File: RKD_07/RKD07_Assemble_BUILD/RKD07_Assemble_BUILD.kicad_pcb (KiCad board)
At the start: 2 copper layers, 233.4 x 200 mm, 172 parts, among them J1 Conn_01x02_Socket, J10 Conn_01x04, J11 TRRS, J12 Conn_01x06, J13 Conn_01x06, J14 Conn_01x02_Socket, J2 Conn_01x24, J3 Conn_01x24, J4 Conn_01x24, J5 Qwiic_RA, J6 Qwiic_RA, J7 Conn_01x06, J8 Conn_01x06, J9 Conn_01x04, M3 Mark, M4 Mark, M5 Mark, M6 Mark, M8 Mark, SW1 SW_Push, SW10 SW_Push, SW11 SW_Push, SW12 SW_Push, SW13 SW_Push, SW14 SW_Push, SW15 SW_Push, SW16 SW_Push, SW17 SW_Push, SW18 SW_Push, SW19 SW_Push, SW2 SW_Push, SW20 SW_Push, SW21 SW_Push, SW22 SW_Push, SW23 SW_Push, SW24 SW_Push, SW25 SW_Push, SW26 SW_Push, SW27 SW_Push, SW28 SW_Push, SW29 SW_Push, SW3 SW_Push, SW30 RotaryEncoder_Switch, SW31 SW_Push, SW4 SW_Push, SW5 SW_Push, SW51 SW_Push, SW52 SW_Push, SW53 SW_Push, SW54 SW_Push, SW55 SW_Push, SW56 SW_Push, SW57 SW_Push, SW58 SW_Push, SW59 SW_Push, SW6 SW_Push, SW60 SW_Push, SW61 SW_Push, SW62 SW_Push, SW63 SW_Push, SW64 SW_Push, SW65 SW_Push, SW66 SW_Push, SW67 SW_Push, SW68 SW_Push, SW69 SW_Push, SW7 SW_Push, SW70 SW_Push, SW71 SW_Push, SW72 SW_Push, SW73 SW_Push, SW74 SW_Push, SW75 SW_Push, SW76 SW_Push, SW77 SW_Push, SW78 SW_Push, SW79 SW_Push, SW8 SW_Push, SW80 SW_Push, SW81 SW_Push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

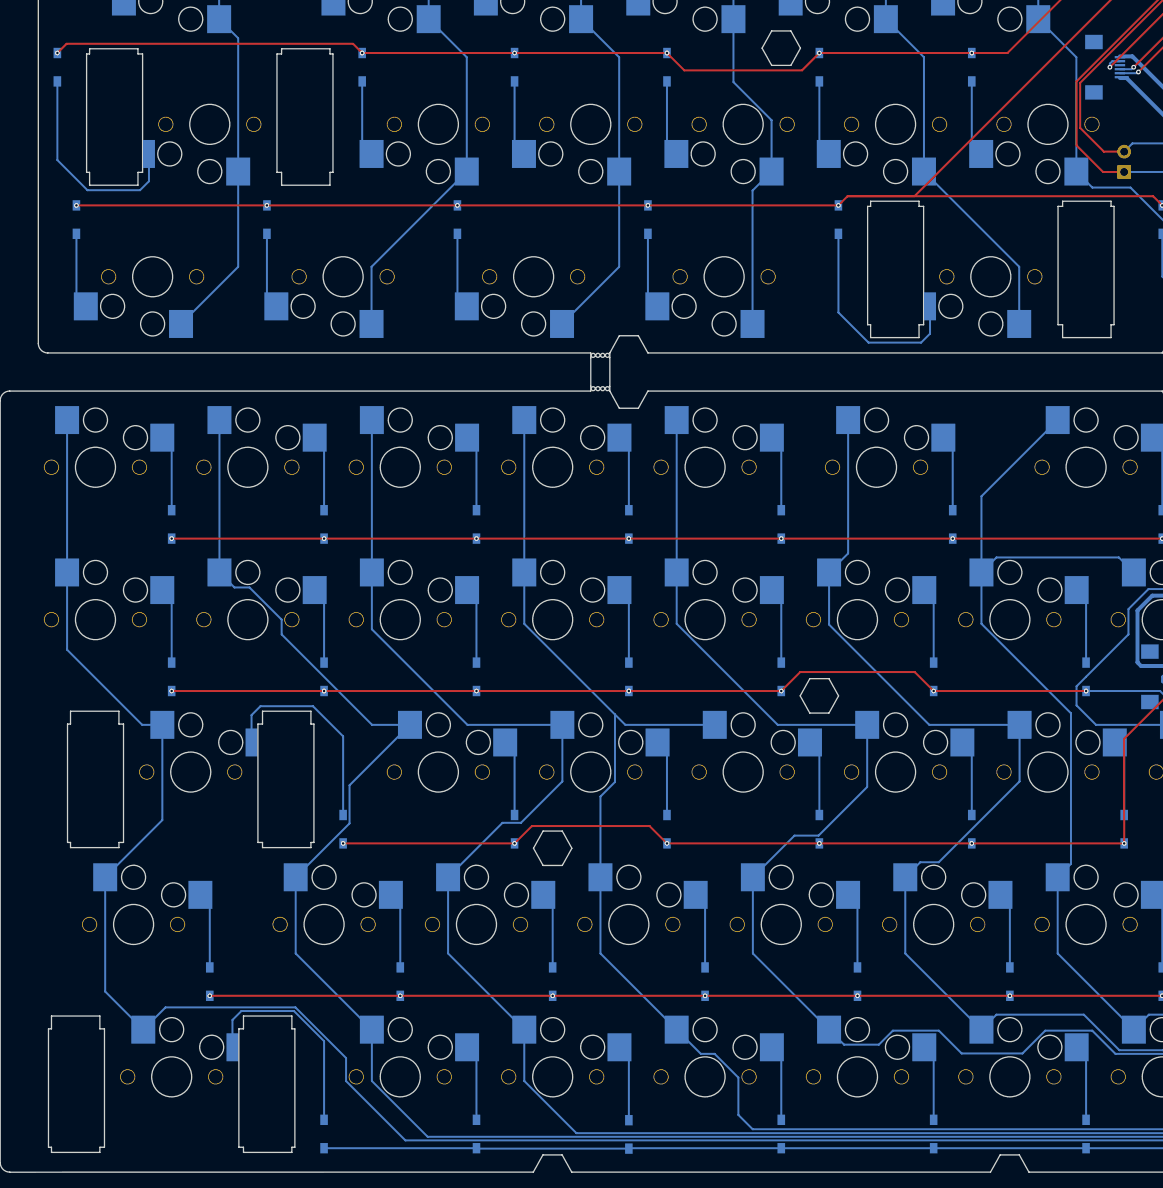
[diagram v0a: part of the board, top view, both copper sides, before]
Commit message: 07 Release調整
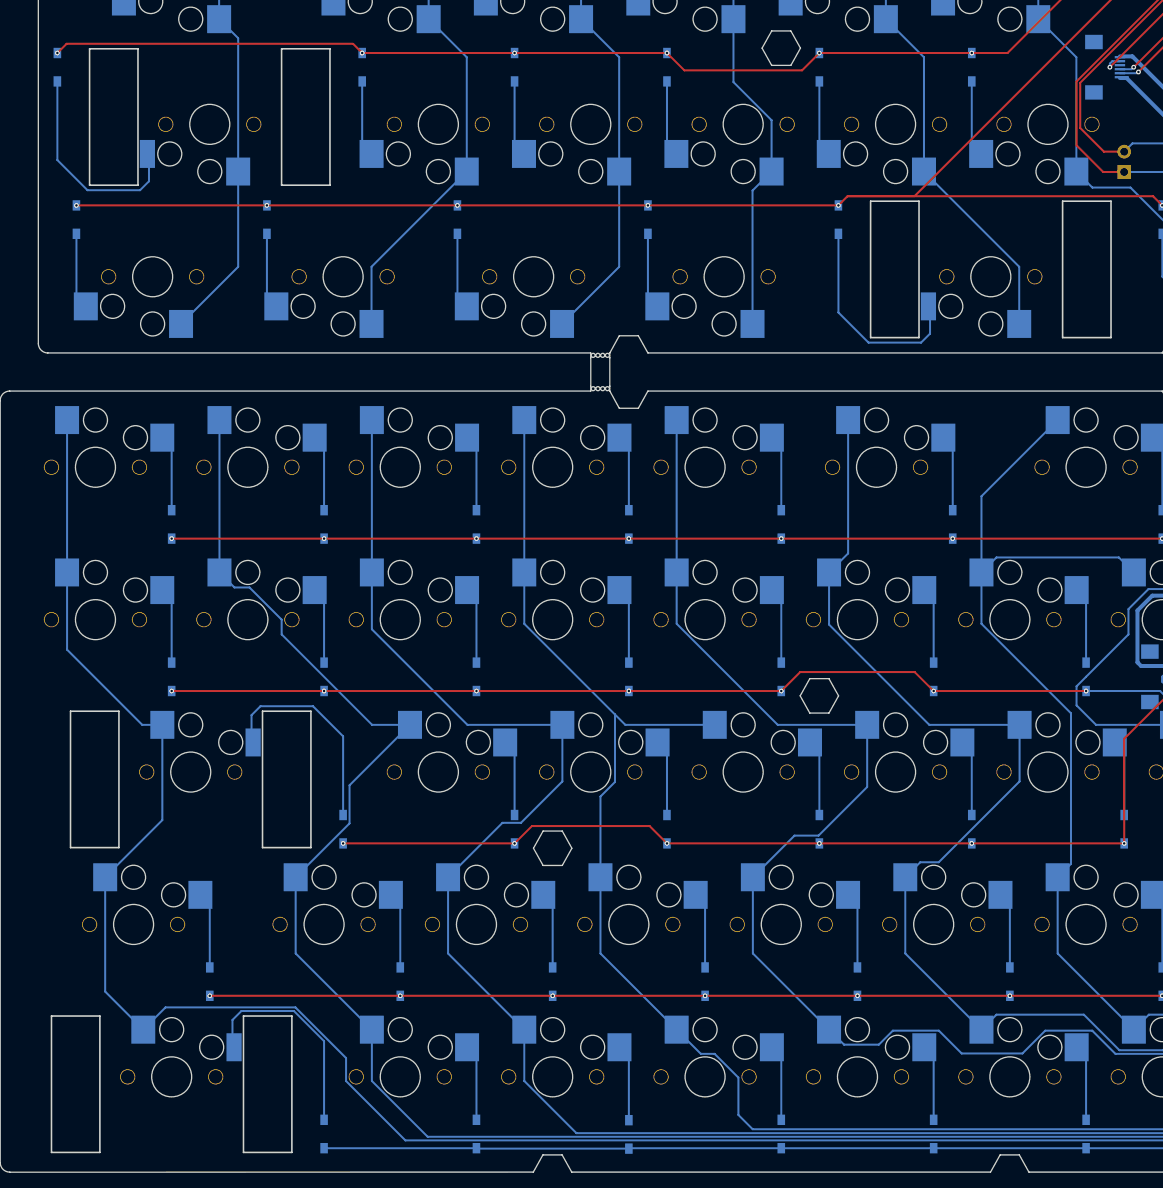
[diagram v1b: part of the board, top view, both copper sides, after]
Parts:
- SW25, SW4, SW86, SW88: footprint Rikkodo_FootPrint:rkd_Asm_ChocV2_Hotswap_2uW -> Rikkodo_FootPrint:rkd_Asm_ChocV2_Hotswap_2u
